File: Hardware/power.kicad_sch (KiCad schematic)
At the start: 77 parts, among them J4 Barrel_Jack_Switch, J8 Conn_01x03, U1 STM32MP157FAD1, U4 STPMIC1

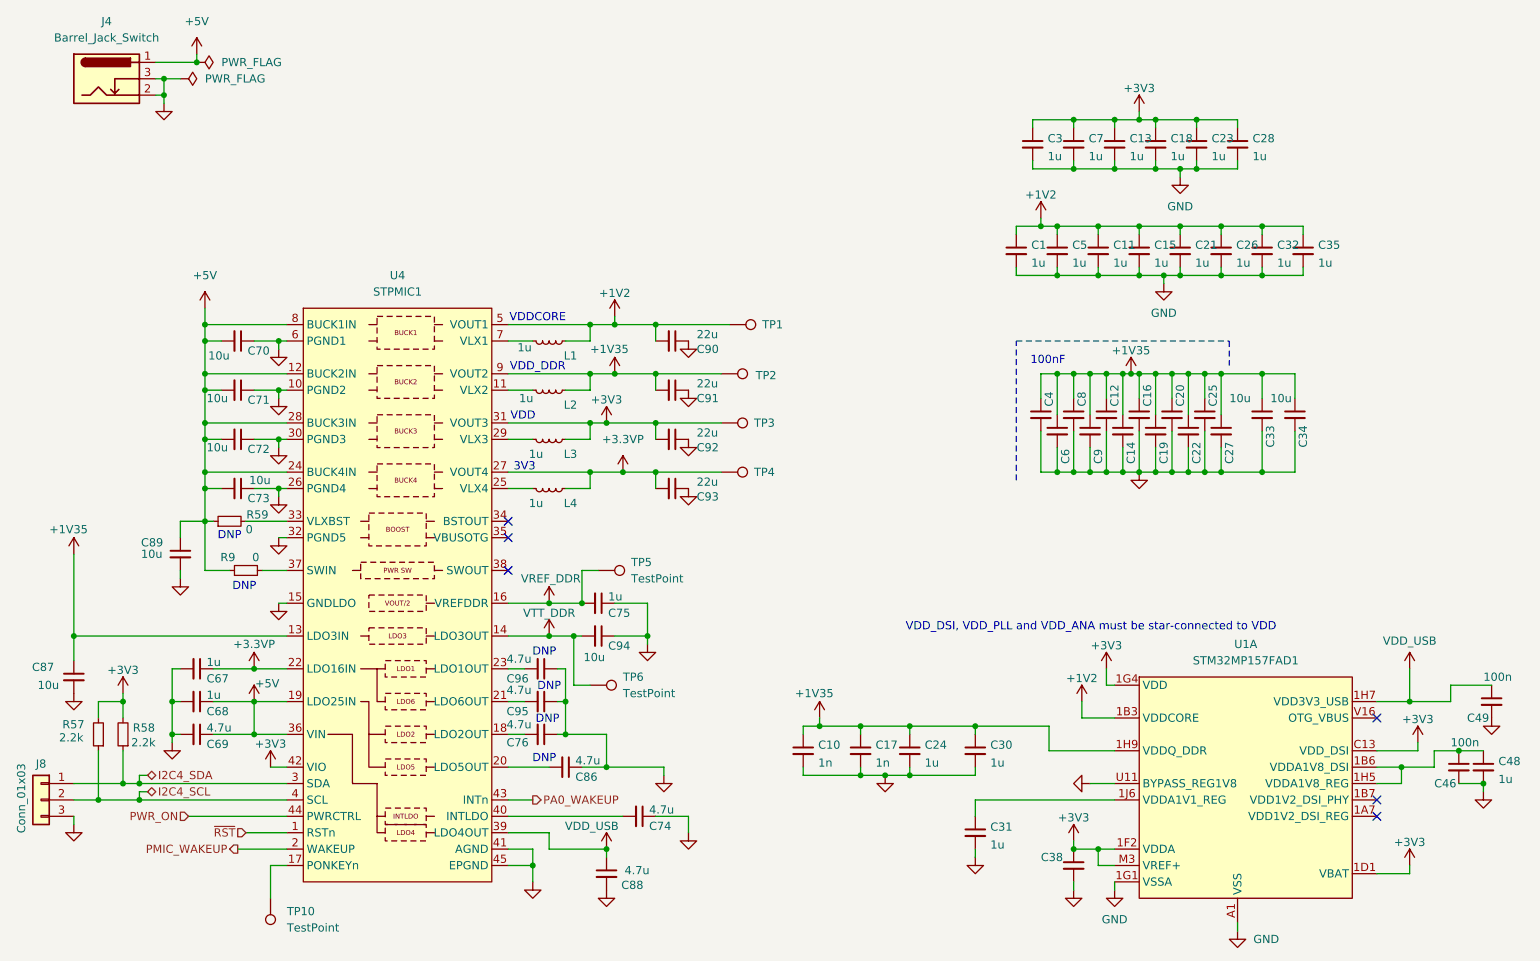
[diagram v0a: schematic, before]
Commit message: First Pass Routing
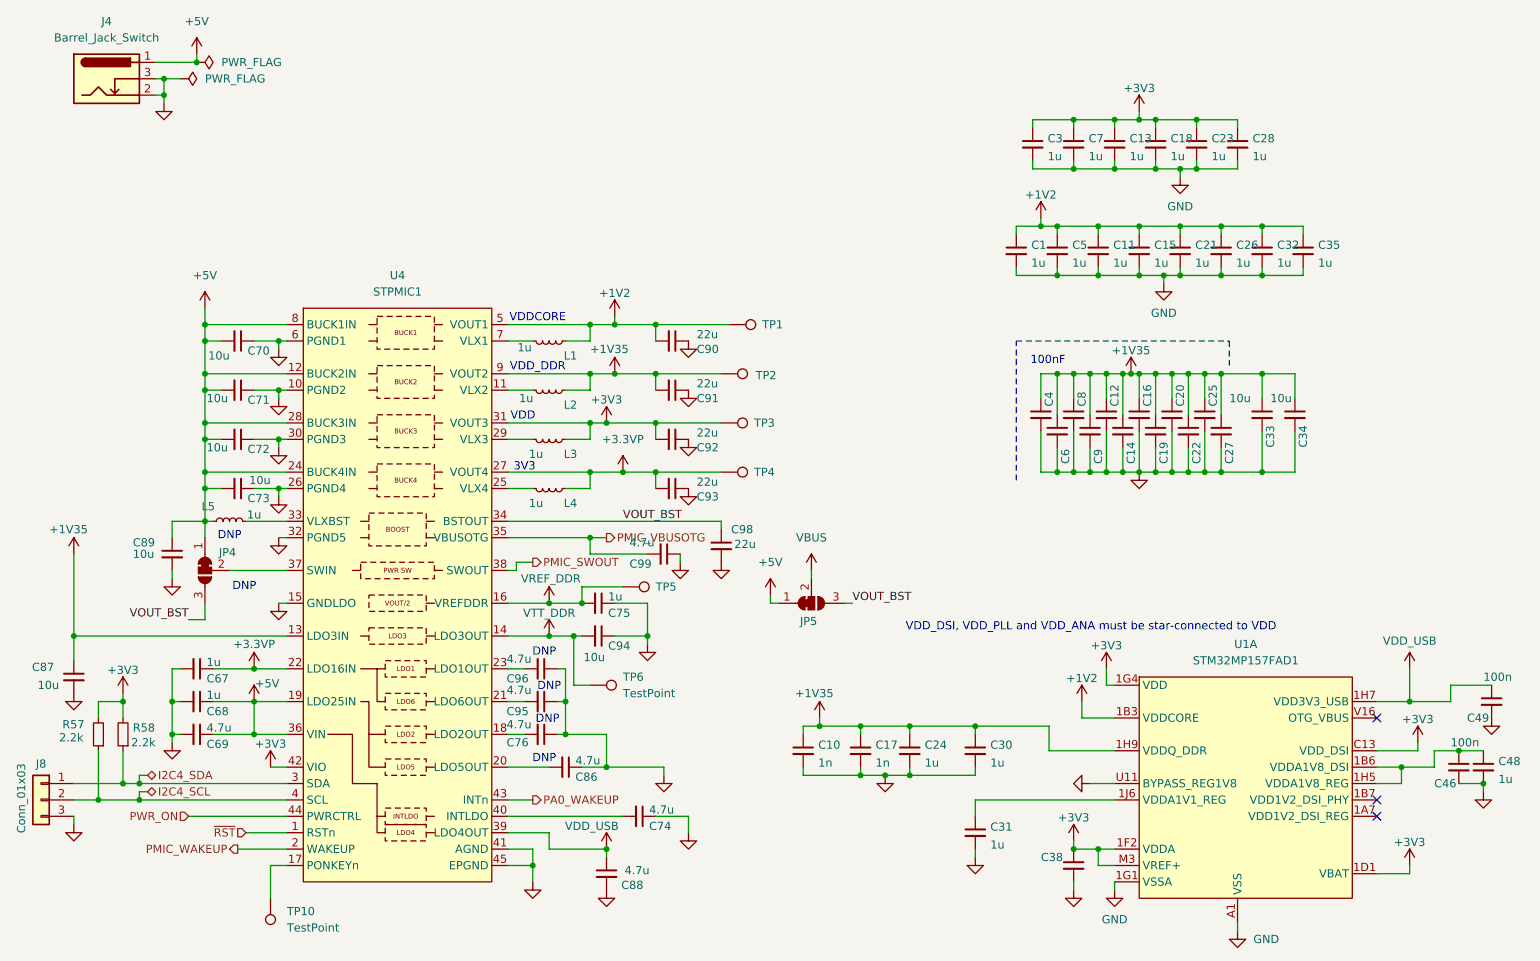
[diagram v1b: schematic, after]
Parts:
- removed R59, R9: 0, Resistor_SMD:R_0402_1005Metric, symbol Device:R_Small
- added C98: 22u, Capacitor_SMD:C_0805_2012Metric, symbol Device:C_Small
- added C99: 4.7u, Capacitor_SMD:C_0402_1005Metric, symbol Device:C_Small
- added JP4, JP5: SolderJumper_3_Bridged12, Jumper:SolderJumper-3_P1.3mm_Bridged2Bar12_Pad1.0x1.5mm, symbol Jumper:SolderJumper_3_Bridged12
- added L5: 1u, Inductor_SMD:L_1008_2520Metric, symbol Device:L_Small
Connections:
- net +5V: now also JP4.1 (A), JP5.1 (A), L5.2
- net GND: now also C98.2, C99.1
- net at U4.37 (SWIN): now also JP4.2 (C)
- net at U4.33 (VLXBST): now also L5.1
- net VOUT_BST: now reaches U4.34 (BSTOUT)
- net VOUT_BST: now also C98.1, JP4.3 (B), JP5.3 (B)
- net PMIC_VBUSOTG: now reaches U4.35 (VBUSOTG)
- net PMIC_VBUSOTG: now also C99.2
- net PMIC_SWOUT: now reaches U4.38 (SWOUT)
- new net VBUS: JP5.2 (C)
- no-connect marks 6 -> 3
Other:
- moved on the sheet: C89, TP5
